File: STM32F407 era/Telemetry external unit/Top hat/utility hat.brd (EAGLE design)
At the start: 65 x 56 mm, 22 parts, among them U1 EEPROM24, U2 SC18IM700IPW,112

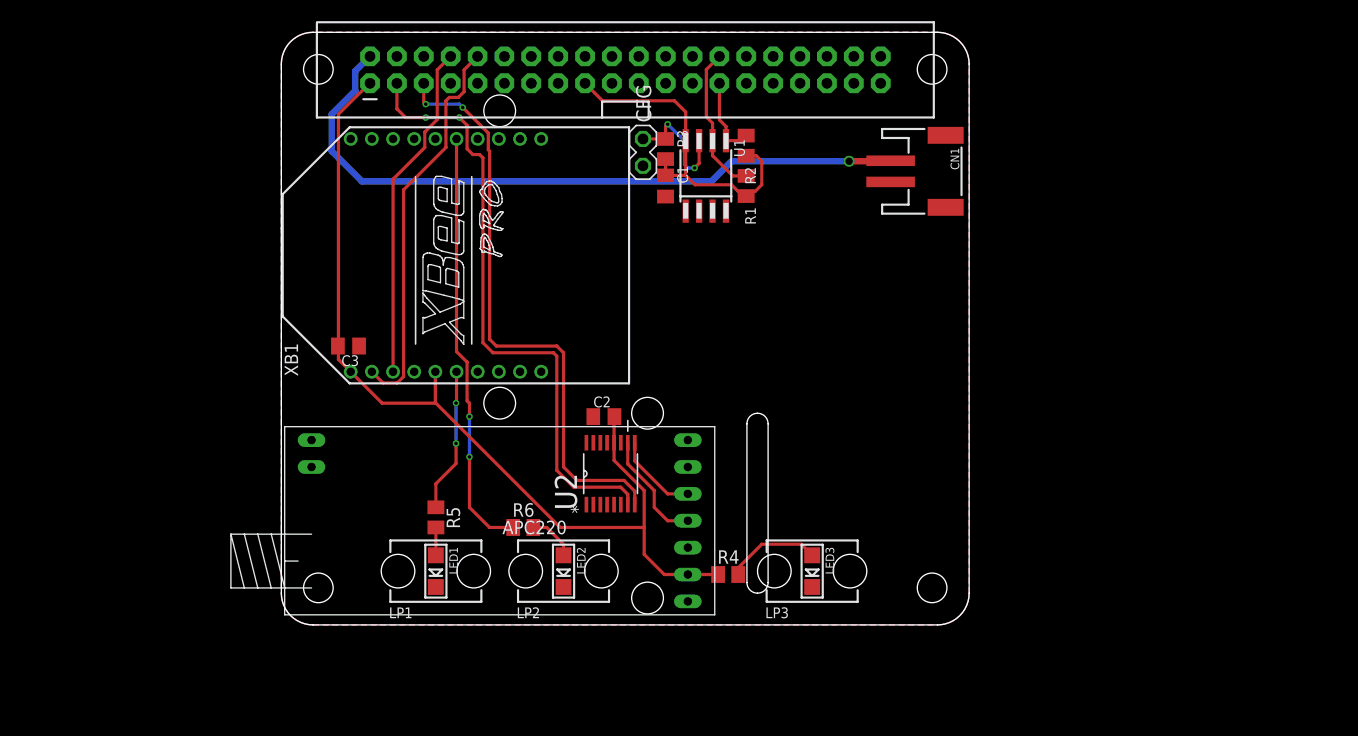
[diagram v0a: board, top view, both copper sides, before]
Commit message: added 5-way CAN splitter and continued work
more work have been done one the laptimer layout
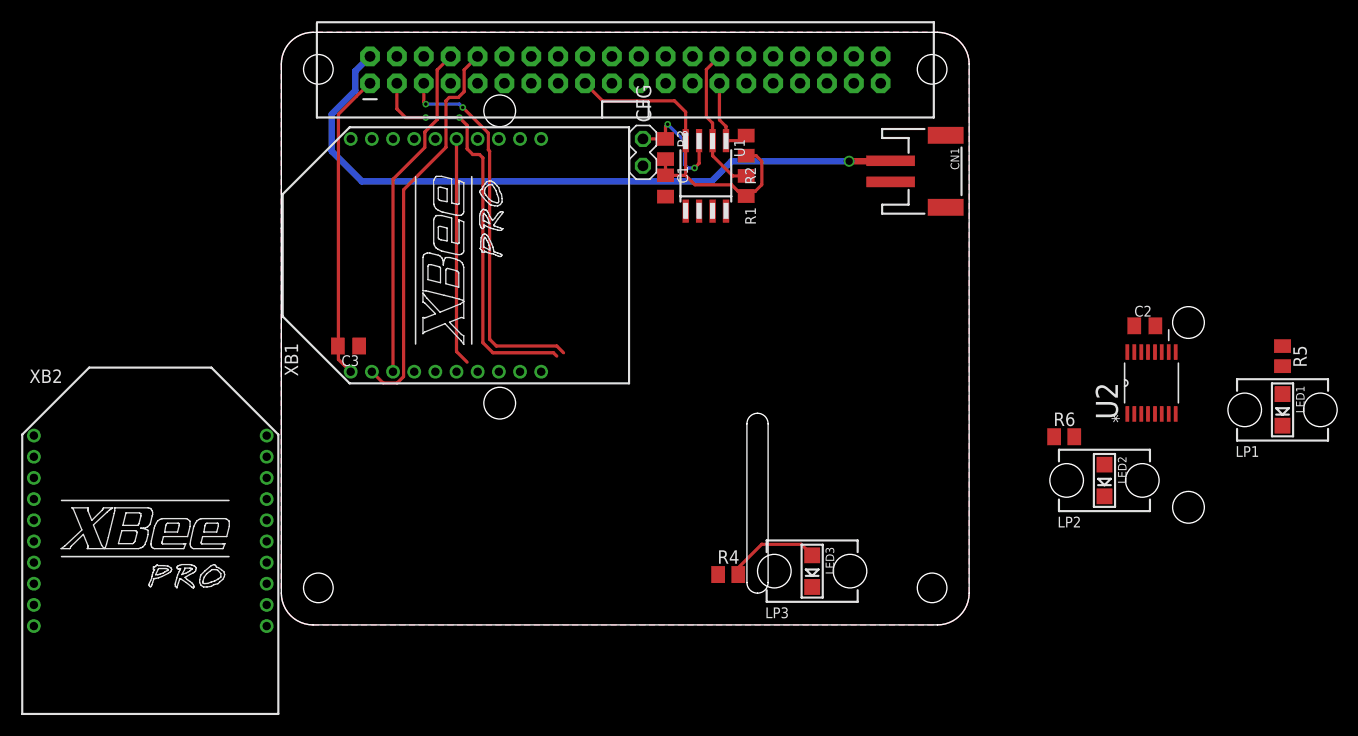
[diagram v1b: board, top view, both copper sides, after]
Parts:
- removed U$1: APC220, APC220:APC220
- added XB2: XBEE-PRO, maxstream:XBEE-PRO
- moved LED1 81.4 mm to (94.6, 20.3)
- moved LP1 81.4 mm to (94.6, 20.3)
- moved R5 81.4 mm to (94.6, 25.4)
- moved R6 51.8 mm to (74.0, 17.8)
- moved U2 51.8 mm to (82.2, 22.9)
- moved C2 51.8 mm to (81.6, 28.3)
- moved LED2 51.8 mm to (77.8, 13.7)
- moved LP2 51.8 mm to (77.8, 13.7)
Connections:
- new net VCC: XB2.1
- net +3V3: now also XB2.5; no longer U$1.VCC
- net GND: now also XB2.10; no longer U$1.GND
- net N$1: now also XB2.3; no longer U$1.RXD
- net N$2: now also XB2.2; no longer U$1.TXD
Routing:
- net +3V3: track 120.5 -> 61.7 mm
- net SCL: track 55.9 -> 36.1 mm
- net SDA: track 58.2 -> 38.7 mm
- net N$5: track 40.2 -> 21.5 mm, vias 2 -> 0
- net N$7: track 13.7 -> 0.00 mm, vias 2 -> 0
- net N$1: track 10.8 -> 0.00 mm
- net N$2: track 8.02 -> 0.00 mm
- net N$6: track 4.56 -> 0.00 mm
- net N$8: track 2.63 -> 0.00 mm
